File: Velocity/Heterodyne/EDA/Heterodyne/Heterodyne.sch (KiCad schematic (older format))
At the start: 37 parts, among them J1 Conn_01x05, J7 Reciever, U1 SA612AD, U2 NE5532DR, U3 MAX7375AXR105, U4 MAX11613, U5 ATmega328PB-AU, Y1 8 MHz

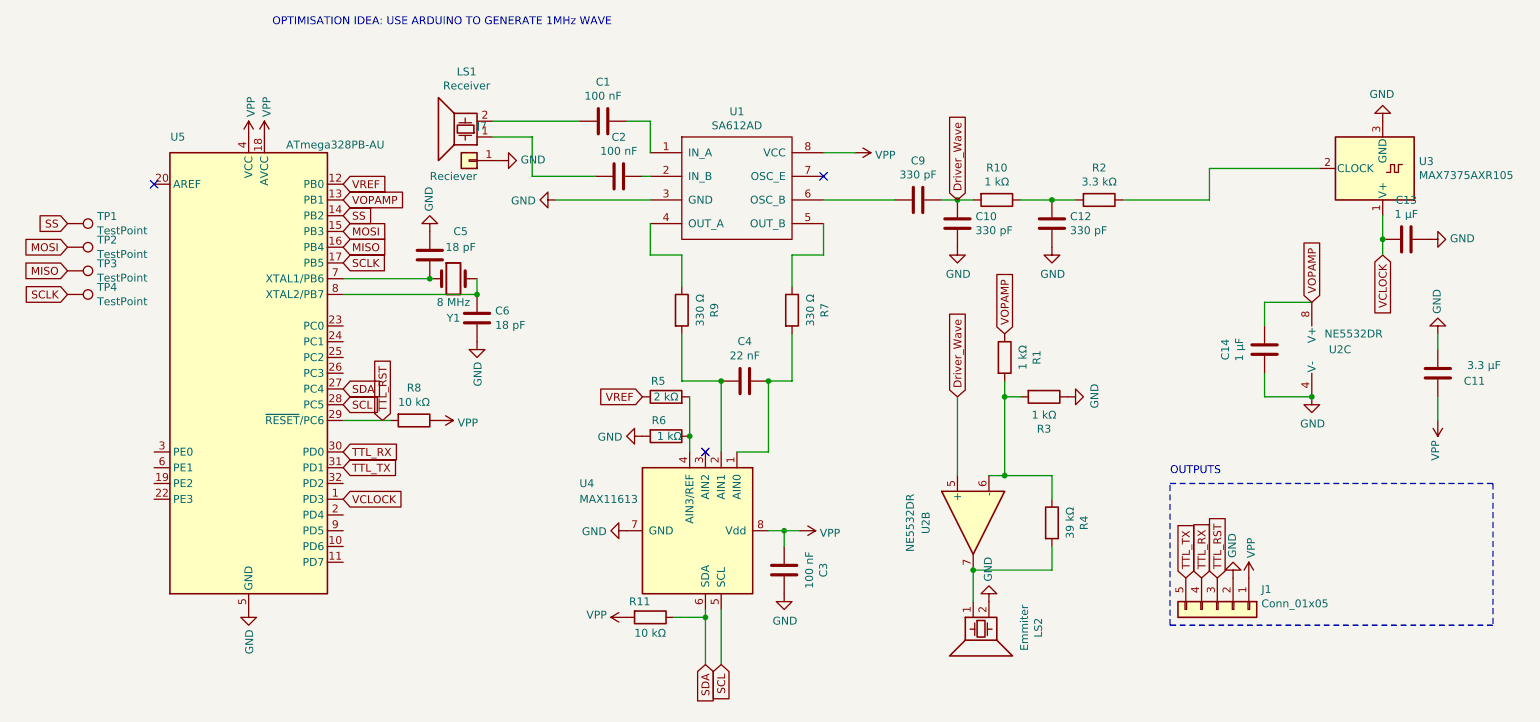
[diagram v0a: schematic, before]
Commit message: finished bosl board rev0.4 layout
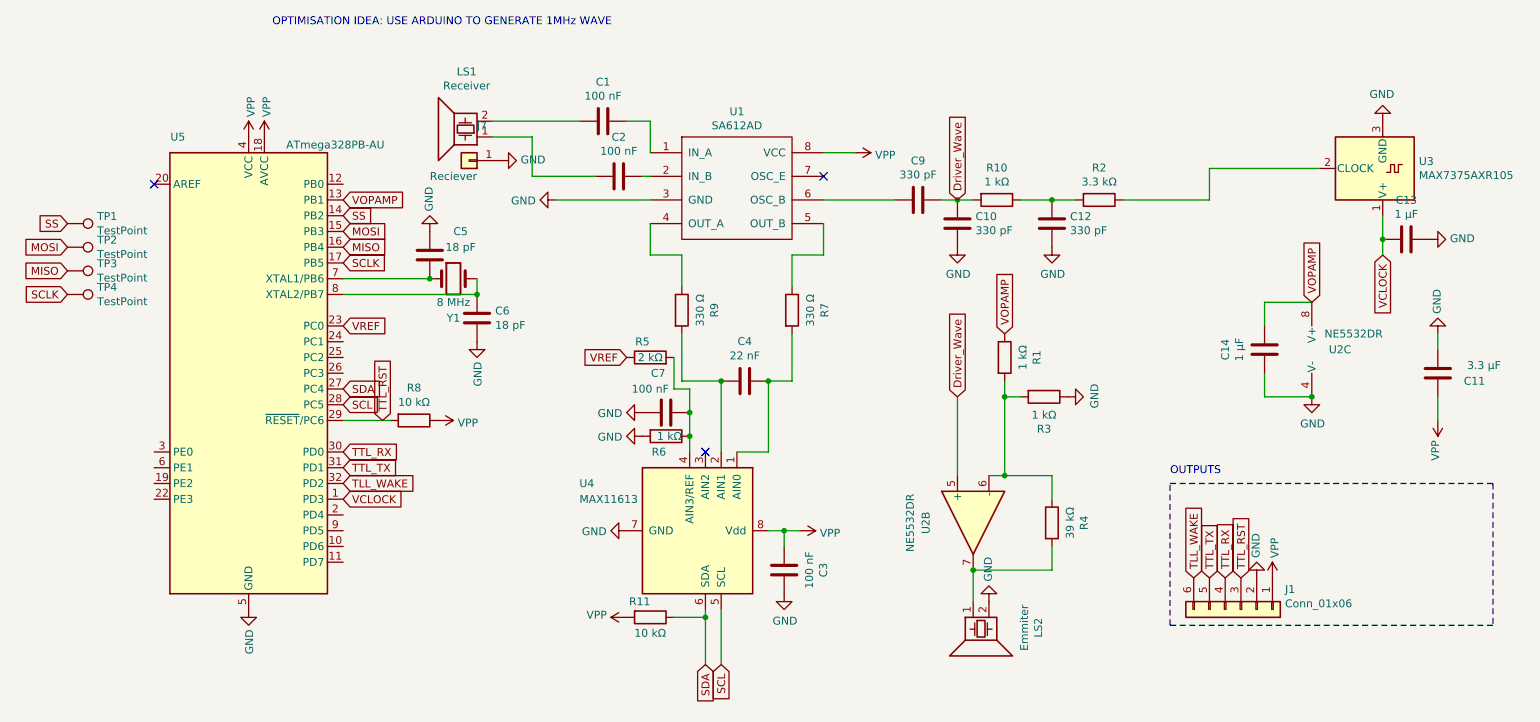
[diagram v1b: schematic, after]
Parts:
- removed J1: Conn_01x05, Connector_PinHeader_2.54mm:PinHeader_1x05_P2.54mm_Vertical, symbol Connector_Generic:Conn_01x05
- added C7: 100 nF, Capacitor_SMD:C_0603_1608Metric_Pad1.05x0.95mm_HandSolder, symbol Heterodyne-rescue:C-Device
- added J1: Conn_01x06, Connector_PinHeader_2.54mm:PinHeader_1x06_P2.54mm_Vertical, symbol Connector_Generic:Conn_01x06
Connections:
- net GND: now also C7.2, J1.2 (Pin_2)
- net TTL_RST: now also J1.3 (Pin_3)
- net TTL_RX: now also J1.4 (Pin_4)
- net TTL_TX: now also J1.5 (Pin_5)
- net VPP: now also J1.1 (Pin_1)
- net VREF: now also U5.23 (PC0); no longer U5.12 (PB0)
- net at R5.2, R6.1, U4.4 (AIN3/REF): now also C7.1
- net TLL_WAKE: now reaches U5.32 (PD2)
- net TLL_WAKE: now also J1.6 (Pin_6)
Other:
- moved on the sheet: R5
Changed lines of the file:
@@
 L Heterodyne-rescue:GND-power #PWR0123
 U 1 1 5E3B45F2
-P 8450 4950
-F 0 "#PWR0123" H 8450 4700 50  0001 C CNN
-F 1 "GND" V 8455 4823 50  0000 R CNN
-F 2 "" H 8450 4950 50  0001 C CNN
-F 3 "" H 8450 4950 50  0001 C CNN
-	1    8450 4950
+P 8600 4950
+F 0 "#PWR0123" H 8600 4700 50  0001 C CNN
+F 1 "GND" V 8605 4823 50  0000 R CNN
+F 2 "" H 8600 4950 50  0001 C CNN
+F 3 "" H 8600 4950 50  0001 C CNN
+	1    8600 4950
 	-1   0    0    1
 $EndComp
@@
 L Heterodyne-rescue:VPP-power #PWR0124
 U 1 1 5E3B49BA
-P 8550 4950
-F 0 "#PWR0124" H 8550 4800 50  0001 C CNN
-F 1 "VPP" V 8565 5076 50  0000 L CNN
-F 2 "" H 8550 4950 50  0001 C CNN
-F 3 "" H 8550 4950 50  0001 C CNN
-	1    8550 4950
+P 8700 4950
+F 0 "#PWR0124" H 8700 4800 50  0001 C CNN
+F 1 "VPP" V 8715 5076 50  0000 L CNN
+F 2 "" H 8700 4950 50  0001 C CNN
+F 3 "" H 8700 4950 50  0001 C CNN
+	1    8700 4950
 	1    0    0    -1
 $EndComp
@@
 U 1 1 5E436A94
 P 4850 4050
-F 0 "R6" V 4750 4050 50  0000 R CNN
+F 0 "R6" V 4950 4050 50  0000 R CNN
 F 1 "1 kΩ" V 4850 4150 50  0000 R CNN
 F 2 "Resistor_SMD:R_0603_1608Metric_Pad1.05x0.95mm_HandSolder" V 4780 4050 50  0001 C CNN
@@
 L Device:R R5
 U 1 1 5E436F78
-P 4850 3800
-F 0 "R5" V 4950 3850 50  0000 C CNN
-F 1 "2 kΩ" V 4850 3800 50  0000 C CNN
-F 2 "Resistor_SMD:R_0603_1608Metric_Pad1.05x0.95mm_HandSolder" V 4780 3800 50  0001 C CNN
-F 3 "~" H 4850 3800 50  0001 C CNN
-	1    4850 3800
+P 4750 3550
+F 0 "R5" V 4850 3600 50  0000 C CNN
+F 1 "2 kΩ" V 4750 3550 50  0000 C CNN
+F 2 "Resistor_SMD:R_0603_1608Metric_Pad1.05x0.95mm_HandSolder" V 4680 3550 50  0001 C CNN
+F 3 "~" H 4750 3550 50  0001 C CNN
+	1    4750 3550
 	0    -1   -1   0
 $EndComp
@@
 Wire Wire Line
 	5650 3700 5500 3700
-Wire Wire Line
-	5000 3800 5000 4050
-Connection ~ 5000 4050
 Wire Wire Line
 	5200 4150 5200 3700
@@
 	1    4600 5200
 	0    -1   -1   0
-$EndComp
-$Comp
-L MCU_Microchip_ATmega:ATmega328PB-AU U5
-U 1 1 5E452B6B
-P 2200 3650
-F 0 "U5" H 1750 5150 50  0000 C CNN
-F 1 "ATmega328PB-AU" H 2750 5100 50  0000 C CNN
-F 2 "Package_QFP:TQFP-32_7x7mm_P0.8mm" H 2200 3650 50  0001 C CIN
-F 3 "http://ww1.microchip.com/downloads/en/DeviceDoc/40001906C.pdf" H 2200 3650 50  0001 C CNN
-	1    2200 3650
-	1    0    0    -1
 $EndComp
 $Comp
@@
 Text GLabel 3050 3950 1    50   Input ~ 0
 TTL_RST
-Text GLabel 8350 4950 1    50   Input ~ 0
+Text GLabel 8500 4950 1    50   Input ~ 0
 TTL_RST
-Text GLabel 8250 4950 1    50   Input ~ 0
+Text GLabel 8400 4950 1    50   Input ~ 0
 TTL_RX
-Text GLabel 8150 4950 1    50   Input ~ 0
+Text GLabel 8300 4950 1    50   Input ~ 0
 TTL_TX
 $Comp
@@
 Text GLabel 7000 3400 1    50   Input ~ 0
 VOPAMP
-$Comp
-L Connector_Generic:Conn_01x05 J1
-U 1 1 5E4B4FBE
-P 8350 5150
-F 0 "J1" V 8222 5430 50  0000 L CNN
-F 1 "Conn_01x05" V 8313 5430 50  0000 L CNN
-F 2 "Connector_PinHeader_2.54mm:PinHeader_1x05_P2.54mm_Vertical" H 8350 5150 50  0001 C CNN
-F 3 "~" H 8350 5150 50  0001 C CNN
-	1    8350 5150
-	0    1    1    0
-$EndComp
 Text Notes 2350 1450 0    50   ~ 0
 OPTIMISATION IDEA: USE ARDUINO TO GENERATE 1MHz WAVE
@@
 $EndComp
 NoConn ~ 1600 2450
-Text GLabel 2800 2450 2    50   Input ~ 0
+Text GLabel 2800 3350 2    50   Input ~ 0
 VREF
-Text GLabel 4700 3800 0    50   Input ~ 0
+Text GLabel 4600 3550 0    50   Input ~ 0
 VREF
+$Comp
+L Connector_Generic:Conn_01x06 J1
+U 1 1 5E9822C7
+P 8500 5150
+F 0 "J1" V 8372 5430 50  0000 L CNN
+F 1 "Conn_01x06" V 8463 5430 50  0000 L CNN
+F 2 "Connector_PinHeader_2.54mm:PinHeader_1x06_P2.54mm_Vertical" H 8500 5150 50  0001 C CNN
+F 3 "~" H 8500 5150 50  0001 C CNN
+	1    8500 5150
+	0    1    1    0
+$EndComp
+Text GLabel 2800 4350 2    50   Input ~ 0
+TLL_WAKE
+$Comp
+L MCU_Microchip_ATmega:ATmega328PB-AU U5
+U 1 1 5E452B6B
+P 2200 3650
+F 0 "U5" H 1750 5150 50  0000 C CNN
+F 1 "ATmega328PB-AU" H 2750 5100 50  0000 C CNN
+F 2 "Package_QFP:TQFP-32_7x7mm_P0.8mm" H 2200 3650 50  0001 C CIN
+F 3 "http://ww1.microchip.com/downloads/en/DeviceDoc/40001906C.pdf" H 2200 3650 50  0001 C CNN
+	1    2200 3650
+	1    0    0    -1
+$EndComp
+Text GLabel 8200 4950 1    50   Input ~ 0
+TLL_WAKE
+$Comp
+L Heterodyne-rescue:C-Device C7
+U 1 1 5E989C6F
+P 4850 3900
+F 0 "C7" V 4600 3850 50  0000 C CNN
+F 1 "100 nF" V 4700 3800 50  0000 C CNN
+F 2 "Capacitor_SMD:C_0603_1608Metric_Pad1.05x0.95mm_HandSolder" H 4888 3750 50  0001 C CNN
+F 3 "~" H 4850 3900 50  0001 C CNN
+	1    4850 3900
+	0    1    1    0
+$EndComp
+$Comp
+L Heterodyne-rescue:GND-power #PWR01
+U 1 1 5E9905FE
+P 4700 3900
+F 0 "#PWR01" H 4700 3650 50  0001 C CNN
+F 1 "GND" V 4705 3773 50  0000 R CNN
+F 2 "" H 4700 3900 50  0001 C CNN
+F 3 "" H 4700 3900 50  0001 C CNN
+	1    4700 3900
+	0    1    1    0
+$EndComp
+Wire Wire Line
+	5000 4050 5000 3900
+Connection ~ 5000 4050
+Wire Wire Line
+	4900 3750 5000 3750
+Wire Wire Line
+	5000 3750 5000 3900
+Connection ~ 5000 3900
+Wire Wire Line
+	4900 3550 4900 3750
 $EndSCHEMATC
